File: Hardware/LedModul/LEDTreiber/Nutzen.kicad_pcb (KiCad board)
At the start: 2 copper layers, 84 x 84 mm, 400 parts, among them J1 Conn_01x01_Pin, J2 Conn_01x01_Pin, J3 Conn_01x01_Pin, J4 Conn_01x01_Pin, J5 Conn_01x01_Pin, U1 TPS92200DxRXL, U2 TVS2700DRV

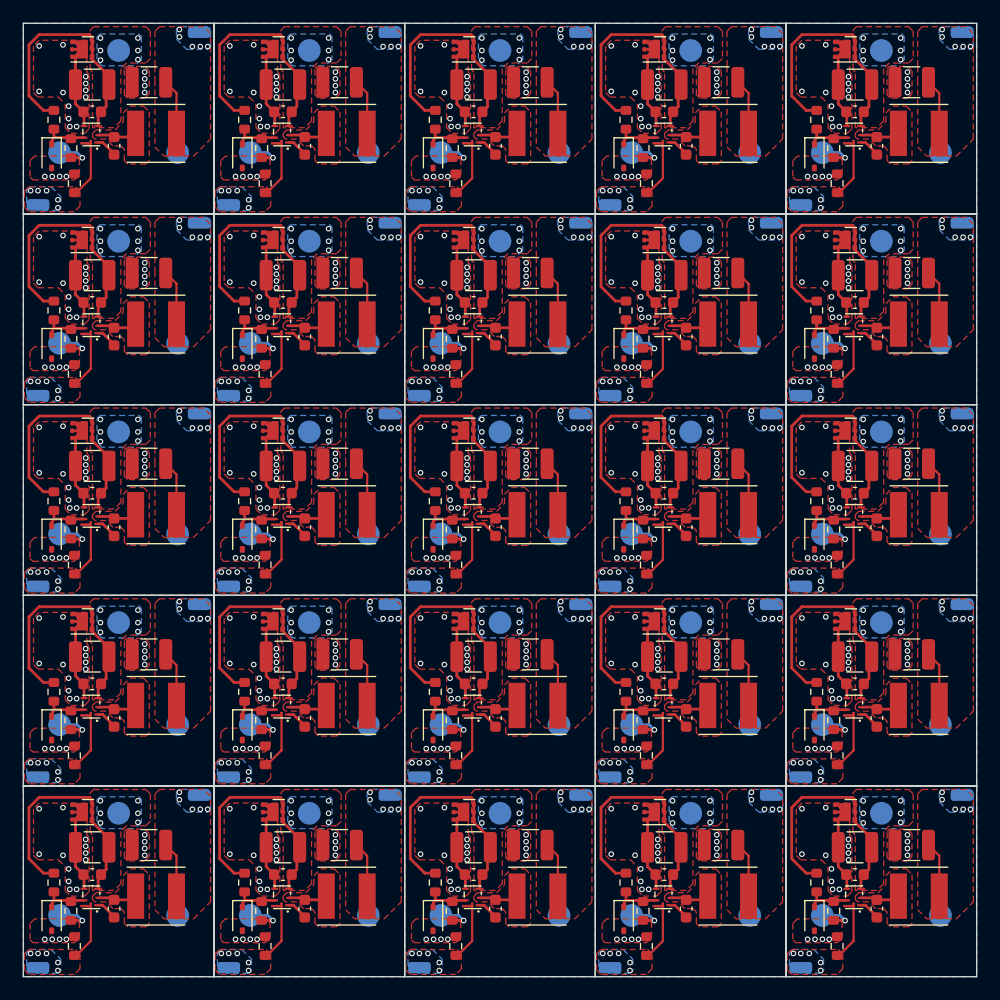
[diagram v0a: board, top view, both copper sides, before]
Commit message: added gerber data
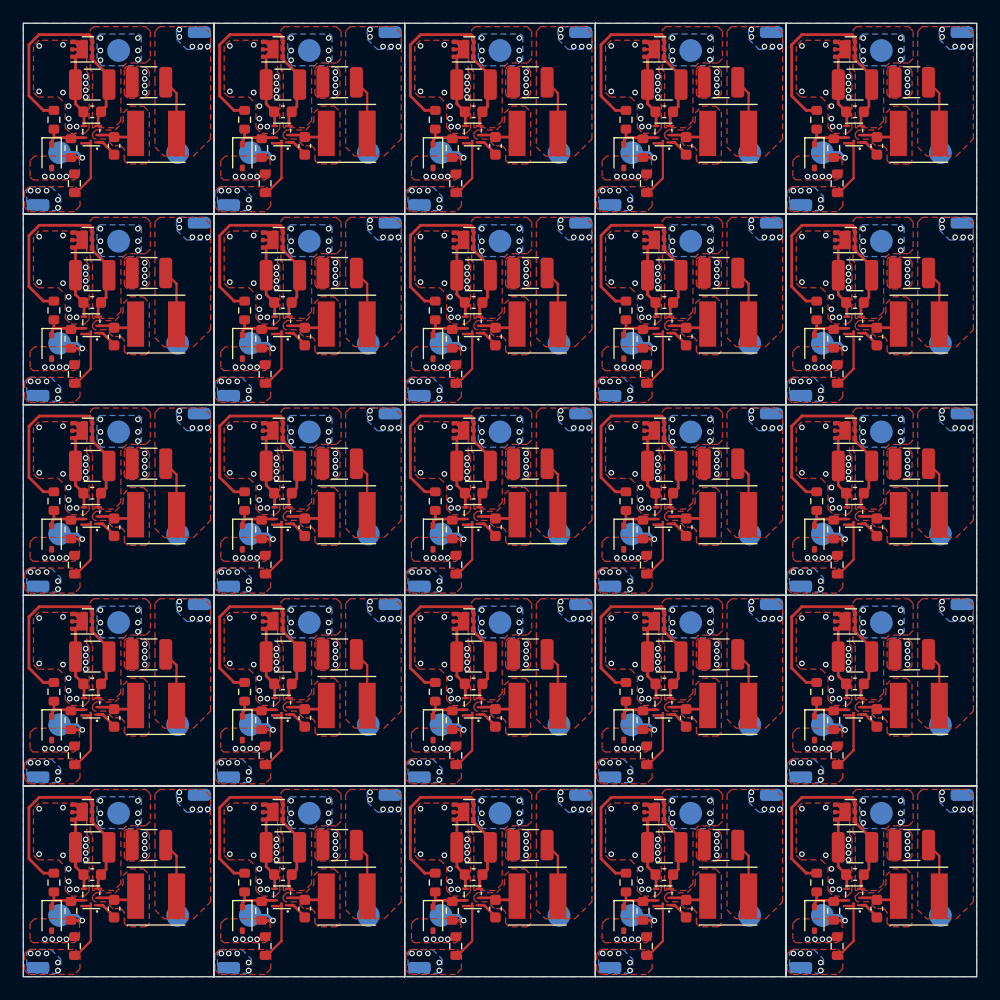
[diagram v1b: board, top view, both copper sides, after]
